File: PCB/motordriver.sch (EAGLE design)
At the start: 6 parts

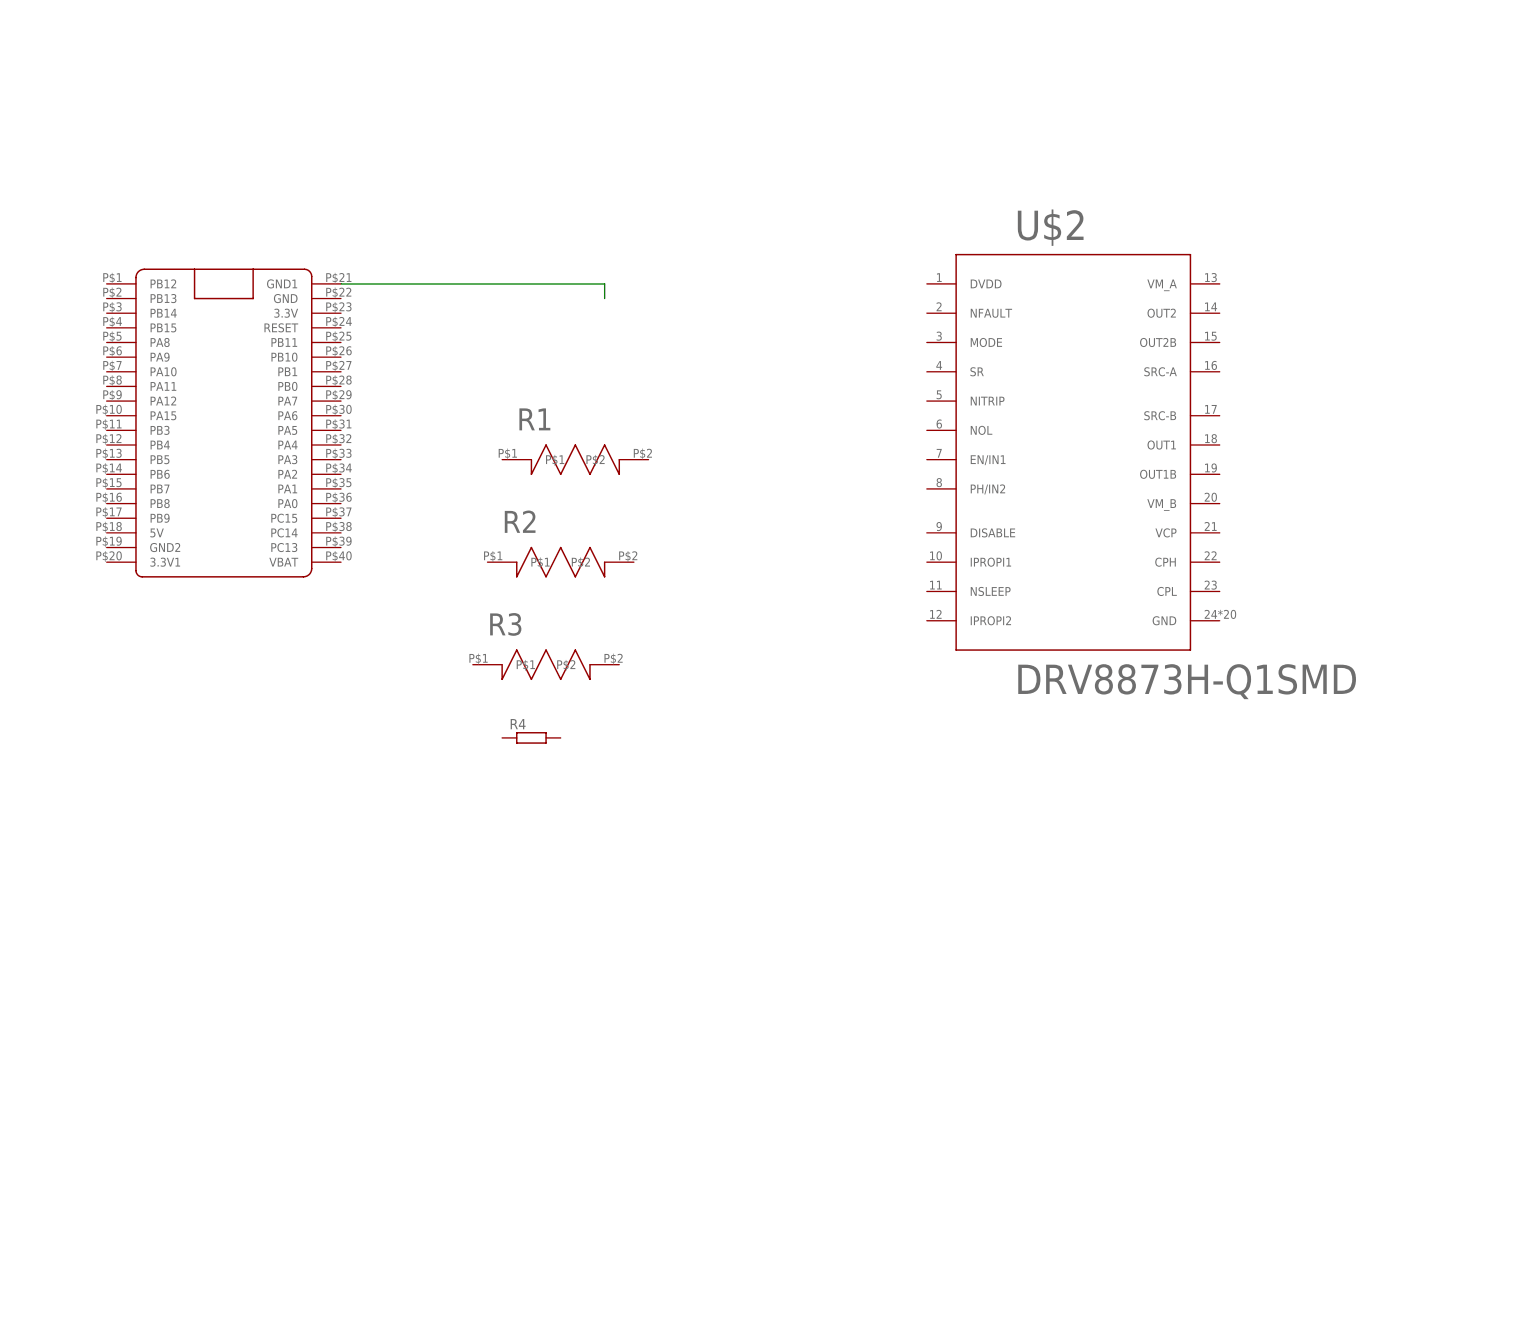
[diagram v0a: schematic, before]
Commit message: work in PCB
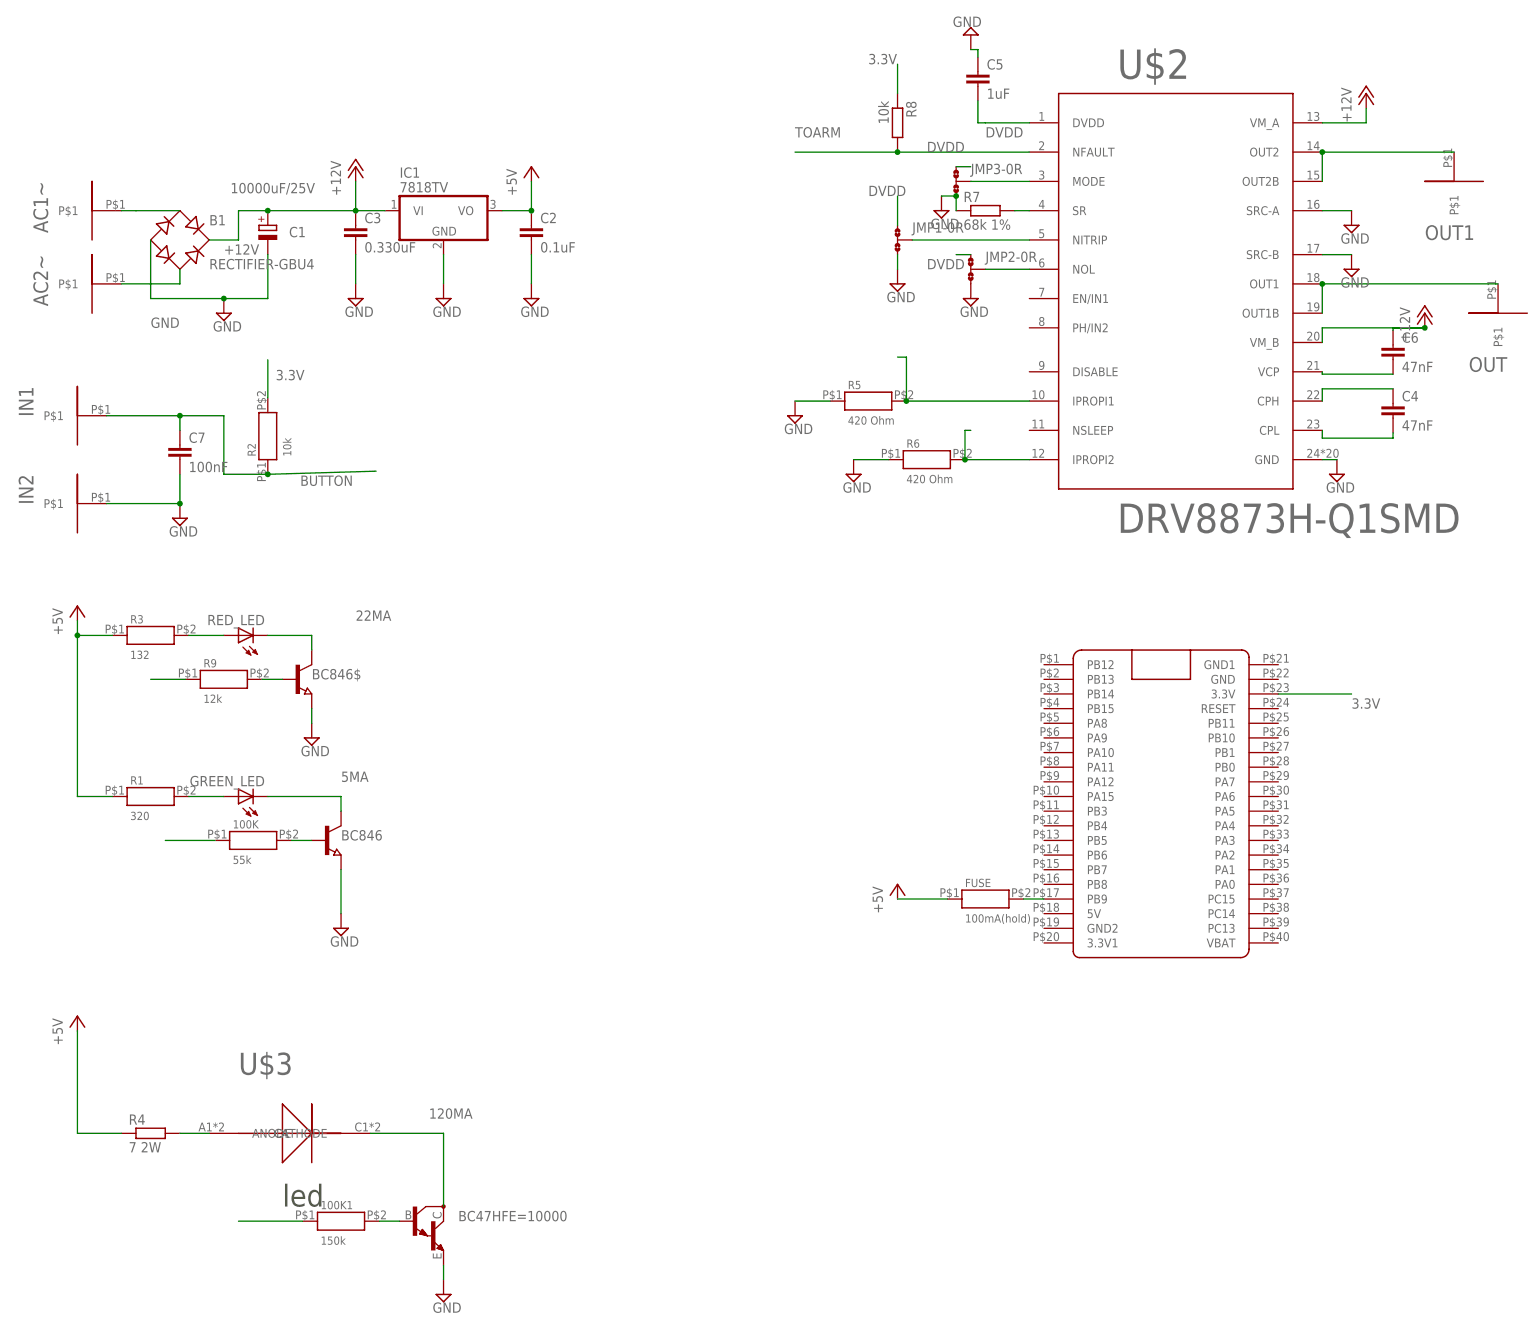
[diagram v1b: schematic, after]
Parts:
- added 100K: 55k, myLibrary:RESISTOR0805_SMD
- added 100K1: 150k, myLibrary:RESISTOR0805_SMD
- added AC1~, AC2~, IN1, IN2, OUT, OUT1: SMDPAD, myLibrary:SMDPAD
- added B1: RECTIFIER-GBU4, rectifier:RECTIFIER-GBU4
- added BC47HFE=10000: MMBTA14LT1, transistor-npn:MMBTA14LT1
- added BC846, BC846$: (no value), semicon-smd-ipc:NPN-TRANSISTOR_SOT23
- added C1: 10000uF/25V, rcl:CPOL-EUE7.5-18
- added C2: 0.1uF, rcl:C-EUC1206
- added C3: 0.330uF, rcl:C-EUC1206
- added C4, C6: 47nF, rcl:C-EUC1206K
- added C5: 1uF, rcl:C-EUC1206K
- added C7: 100nF, rcl:C-EUC1206
- added FUSE: 100mA(hold), myLibrary:RESISTOR0805_SMD
- added GREEN_LED, RED_LED: (no value), led:LEDCHIPLED_0805
- added IC1: 7818TV, linear:7818TV
- added JMP1, JMP2, JMP3: 0R-JUMPA, jump-0r-smd:0R-JUMPA
- added R5, R6: 420 Ohm, myLibrary:RESISTOR0805_SMD
- added R7: 68k 1%, resistor:R-EU_R0805
- added R8: 10k, resistor:R-EU_R0805
- added R9: 12k, myLibrary:RESISTOR0805_SMD
- added U$3: POWER_LED, myLibrary:POWER_LED
- R1: value (none) -> 320
- R2: value (none) -> 10k
- R3: value (none) -> 132
- R4: value (none) -> 7 2W; device eagle-ltspice:R -> resistor:R-EU_R1210
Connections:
- new net +12V: B1.+, C1.+, C3.1, C6.1, IC1.VI, U$2.VM_A, U$2.VM_B
- new net +5V: C2.1, FUSE.P$1, IC1.VO, R1.P$1, R3.P$1, R4.1
- new net 120MA: BC47HFE=10000.C, U$3.CATHODE
- new net 22MA: BC846$.C, RED_LED.C
- new net 3.3V: R2.P$2, R8.1, U$1.3.3V
- new net 5MA: BC846.C, GREEN_LED.C
- new net BUTTON: C7.1, IN1.P$1, R2.P$1
- new net DVDD: C5.2, JMP1-0R.1, JMP2-0R.1, JMP3-0R.1, U$2.DVDD
- new net GND: B1.-, BC47HFE=10000.E, BC846$.E, BC846.E, C1.-, C2.2, C3.2, C5.1, C7.2, IC1.GND, IN2.P$1, JMP1-0R.3, JMP2-0R.3, JMP3-0R.3, R5.P$1, R6.P$1, R7.1, U$2.GND, U$2.SRC-A, U$2.SRC-B
- new net N$10: R7.2, U$2.SR
- new net N$11: C6.2, U$2.VCP
- new net N$12: OUT1.P$1, U$2.OUT2, U$2.OUT2B
- new net N$13: OUT.P$1, U$2.OUT1, U$2.OUT1B
- new net N$14: R3.P$2, RED_LED.A
- new net N$15: GREEN_LED.A, R1.P$2
- new net N$18: BC846$.B, R9.P$2
- new net N$19: R9.P$1
- new net N$2: AC2~.P$1, B1.AC2
- new net N$20: 100K.P$2, BC846.B
- new net N$21: 100K.P$1
- new net N$23: R4.2, U$3.ANODE
- new net N$24: 100K1.P$2, BC47HFE=10000.B
- new net N$25: 100K1.P$1
- new net N$26: FUSE.P$2, U$1.PB9
- new net N$3: C4.1, U$2.CPH
- new net N$4: C4.2, U$2.CPL
- new net N$5: JMP2-0R.2, U$2.NOL
- new net N$6: R6.P$2, U$2.IPROPI2
- new net N$7: R5.P$2, U$2.IPROPI1
- new net N$8: JMP1-0R.2, U$2.NITRIP
- new net N$9: JMP3-0R.2, U$2.MODE
- new net TOARM: R8.2, U$2.NFAULT
- net N$1: now also AC1~.P$1, B1.AC1; no longer U$1.GND1
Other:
- moved on the sheet: R4, U$2
